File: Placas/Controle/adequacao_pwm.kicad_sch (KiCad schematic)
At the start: 9 parts, among them Q3 BC337, U19 H11L1

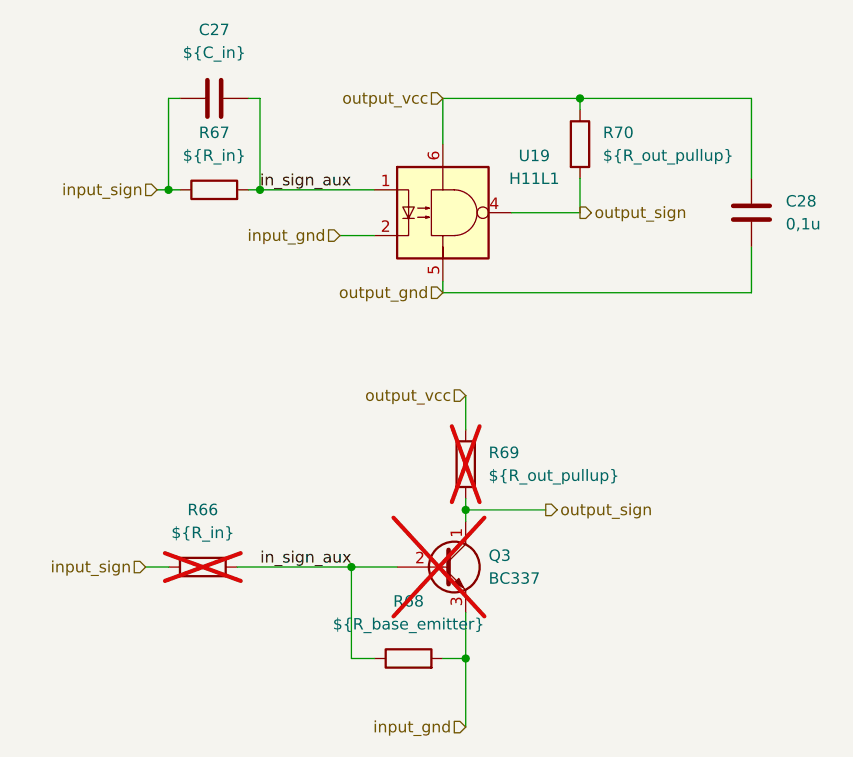
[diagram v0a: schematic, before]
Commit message: Criação de novas pastas com código em C e Matlab
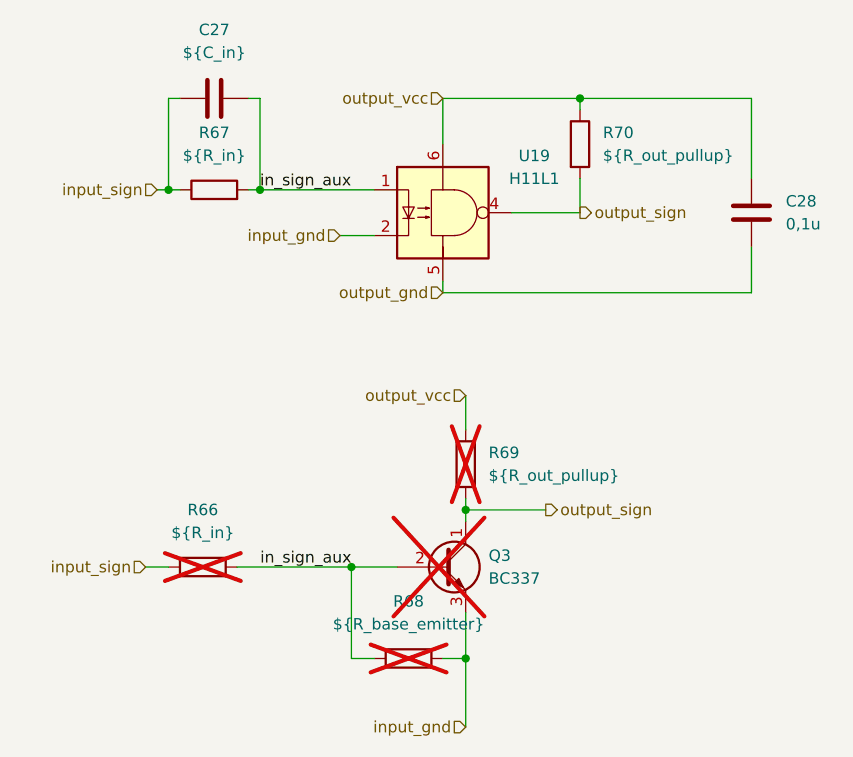
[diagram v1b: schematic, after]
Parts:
- R68: now not fitted
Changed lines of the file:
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@@
 		(in_bom yes)
 		(on_board yes)
-		(dnp no)
+		(dnp yes)
 		(fields_autoplaced yes)
 		(property "Reference" "R68"
